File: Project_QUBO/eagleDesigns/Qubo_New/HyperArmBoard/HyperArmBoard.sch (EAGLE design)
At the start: 16 parts, among them U1 BME280

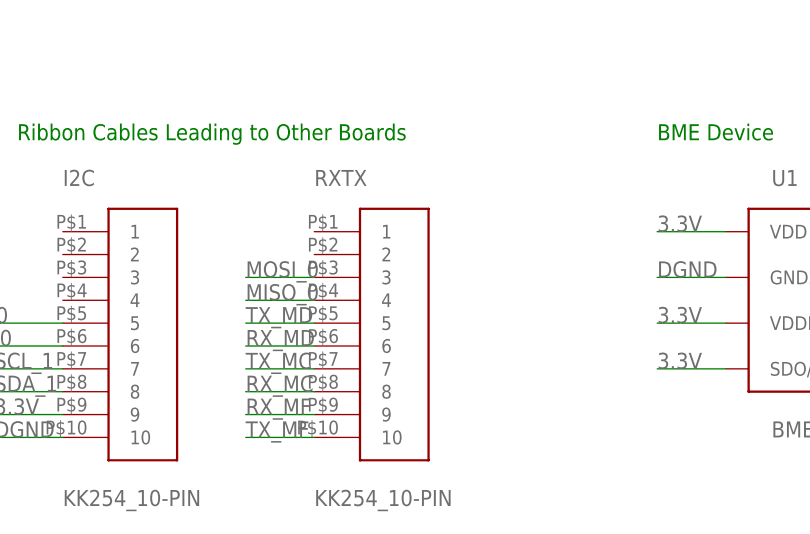
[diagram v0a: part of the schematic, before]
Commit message: changes to hyperarm and power board
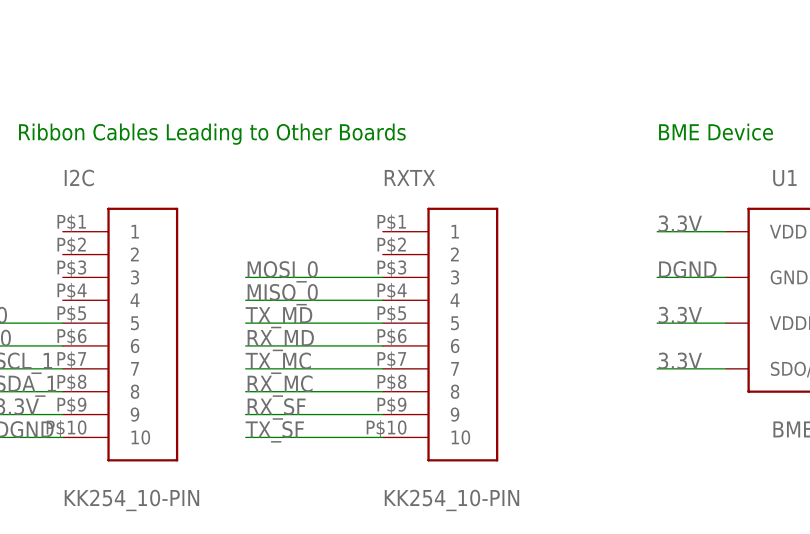
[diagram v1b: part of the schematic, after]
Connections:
- net RX_MF: no longer RXTX.9
- net RX_SF: now also RXTX.9
- net TX_MF: no longer RXTX.10
- net TX_SF: now also RXTX.10
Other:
- moved on the sheet: RXTX
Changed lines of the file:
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@@
 <attribute name="NAME" x="48.26" y="152.4" size="1.778" layer="95"/>
 </instance>
-<instance part="RXTX" gate="G$1" x="167.64" y="33.02" smashed="yes">
-<attribute name="NAME" x="160.02" y="48.26" size="1.778" layer="95"/>
-<attribute name="VALUE" x="160.02" y="12.7" size="1.778" layer="96"/>
+<instance part="RXTX" gate="G$1" x="175.26" y="33.02" smashed="yes">
+<attribute name="NAME" x="167.64" y="48.26" size="1.778" layer="95"/>
+<attribute name="VALUE" x="167.64" y="12.7" size="1.778" layer="96"/>
 </instance>
 </instances>
@@
 <label x="109.22" y="144.78" size="1.778" layer="95"/>
 </segment>
-<segment>
-<pinref part="RXTX" gate="G$1" pin="9"/>
-<wire x1="160.02" y1="22.86" x2="152.4" y2="22.86" width="0.1524" layer="91"/>
-<label x="152.4" y="22.86" size="1.778" layer="95"/>
-</segment>
 </net>
 <net name="TX_MF" class="0">
@@
 <label x="109.22" y="139.7" size="1.778" layer="95"/>
 </segment>
-<segment>
-<pinref part="RXTX" gate="G$1" pin="10"/>
-<wire x1="160.02" y1="20.32" x2="152.4" y2="20.32" width="0.1524" layer="91"/>
-<label x="152.4" y="20.32" size="1.778" layer="95"/>
-</segment>
 </net>
 <net name="3.3V" class="0">
@@
 <segment>
 <pinref part="RXTX" gate="G$1" pin="8"/>
-<wire x1="160.02" y1="25.4" x2="152.4" y2="25.4" width="0.1524" layer="91"/>
+<wire x1="167.64" y1="25.4" x2="152.4" y2="25.4" width="0.1524" layer="91"/>
 <label x="152.4" y="25.4" size="1.778" layer="95"/>
 </segment>
@@
 <segment>
 <pinref part="RXTX" gate="G$1" pin="7"/>
-<wire x1="160.02" y1="27.94" x2="152.4" y2="27.94" width="0.1524" layer="91"/>
+<wire x1="167.64" y1="27.94" x2="152.4" y2="27.94" width="0.1524" layer="91"/>
 <label x="152.4" y="27.94" size="1.778" layer="95"/>
 </segment>
@@
 <label x="236.22" y="129.54" size="1.778" layer="95"/>
 </segment>
+<segment>
+<pinref part="RXTX" gate="G$1" pin="9"/>
+<wire x1="167.64" y1="22.86" x2="152.4" y2="22.86" width="0.1524" layer="91"/>
+<label x="152.4" y="22.86" size="1.778" layer="95"/>
+</segment>
 </net>
 <net name="TX_SF" class="0">
@@
 <label x="236.22" y="124.46" size="1.778" layer="95"/>
 </segment>
+<segment>
+<pinref part="RXTX" gate="G$1" pin="10"/>
+<wire x1="167.64" y1="20.32" x2="152.4" y2="20.32" width="0.1524" layer="91"/>
+<label x="152.4" y="20.32" size="1.778" layer="95"/>
+</segment>
 </net>
 <net name="RX_MD" class="0">
@@
 <segment>
 <pinref part="RXTX" gate="G$1" pin="6"/>
-<wire x1="160.02" y1="30.48" x2="152.4" y2="30.48" width="0.1524" layer="91"/>
+<wire x1="167.64" y1="30.48" x2="152.4" y2="30.48" width="0.1524" layer="91"/>
 <label x="152.4" y="30.48" size="1.778" layer="95"/>
 </segment>
@@
 <segment>
 <pinref part="RXTX" gate="G$1" pin="5"/>
-<wire x1="160.02" y1="33.02" x2="152.4" y2="33.02" width="0.1524" layer="91"/>
+<wire x1="167.64" y1="33.02" x2="152.4" y2="33.02" width="0.1524" layer="91"/>
 <label x="152.4" y="33.02" size="1.778" layer="95"/>
 </segment>
@@
 <segment>
 <pinref part="RXTX" gate="G$1" pin="4"/>
-<wire x1="160.02" y1="35.56" x2="152.4" y2="35.56" width="0.1524" layer="91"/>
+<wire x1="167.64" y1="35.56" x2="152.4" y2="35.56" width="0.1524" layer="91"/>
 <label x="152.4" y="35.56" size="1.778" layer="95"/>
 </segment>
@@
 <segment>
 <pinref part="RXTX" gate="G$1" pin="3"/>
-<wire x1="160.02" y1="38.1" x2="152.4" y2="38.1" width="0.1524" layer="91"/>
+<wire x1="167.64" y1="38.1" x2="152.4" y2="38.1" width="0.1524" layer="91"/>
 <label x="152.4" y="38.1" size="1.778" layer="95"/>
 </segment>
